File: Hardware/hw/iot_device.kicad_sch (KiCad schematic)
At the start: 38 parts, among them J2 USB4085-GF-A_REVA4, J4 Conn_01x04_Pin, J7 Conn_01x02_Pin, Q1 PMOS, Q7 PMOS, SW1 SW_Push, SW2 SW_Push, U1 ESP32-C6-WROOM-1, U2 RV-3028-C7, U5 TPS63001, U9 USBLC6-4SC6

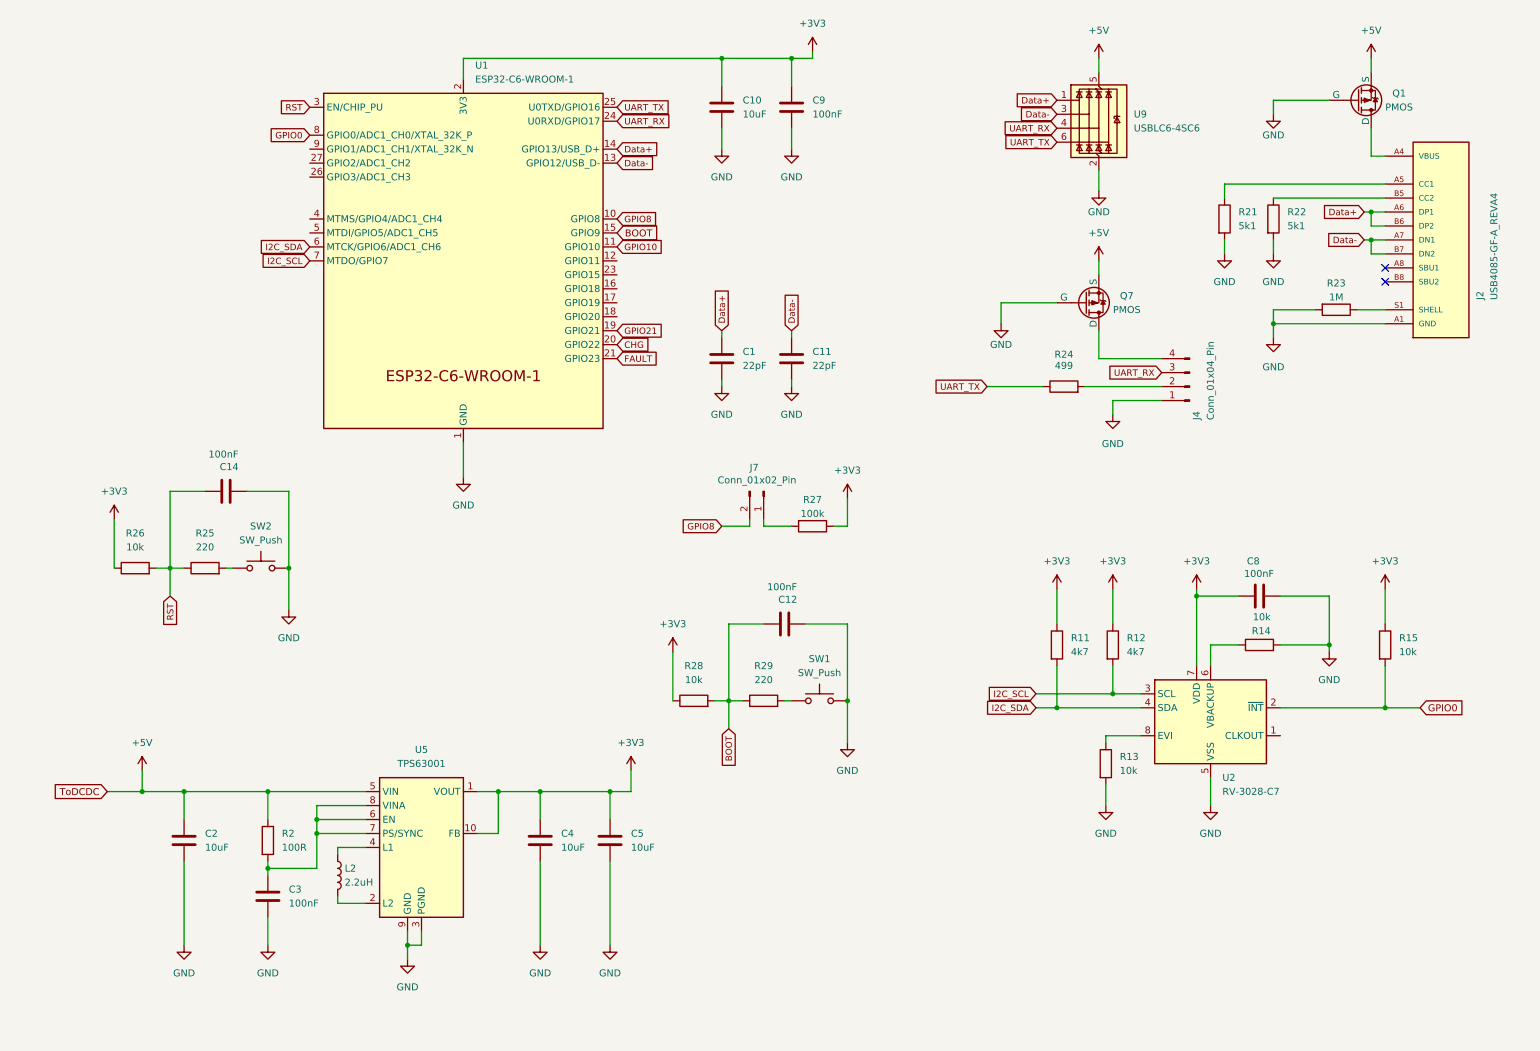
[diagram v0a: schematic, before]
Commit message: Sensors update
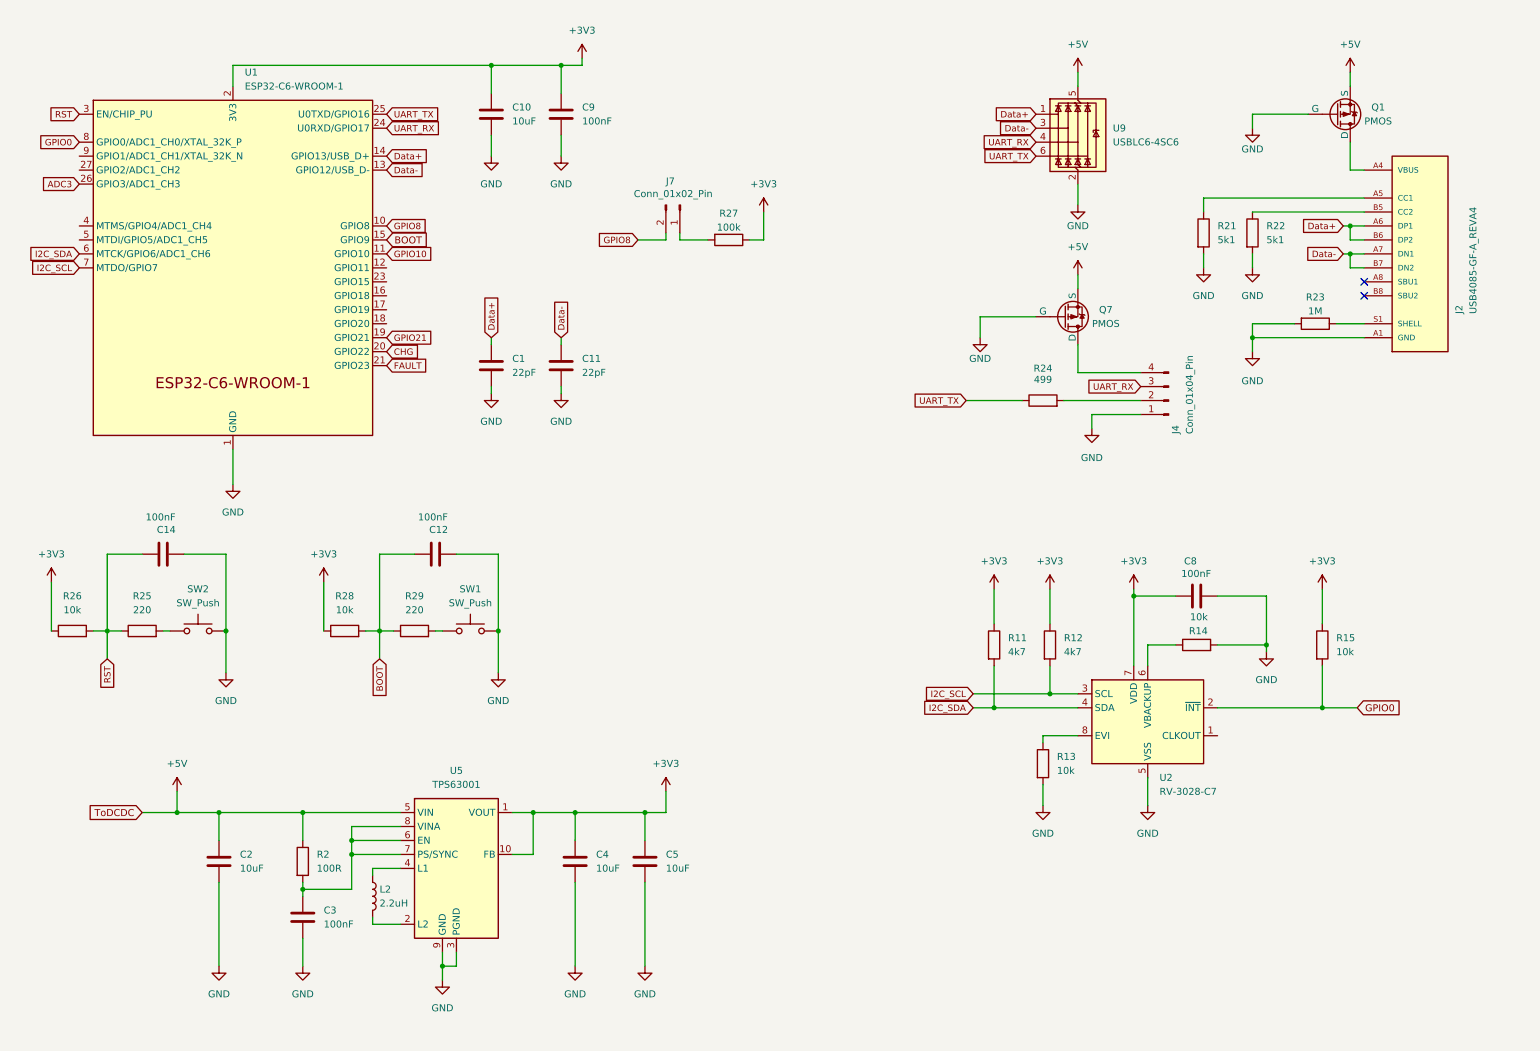
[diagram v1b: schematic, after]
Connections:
- net ADC3: now reaches U1.26 (GPIO3/ADC1_CH3)
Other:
- moved on the sheet: C1, C10, C11, C12, C14, C2, C3, C4, C5, C8, C9, J2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

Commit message: Hardware v1.0
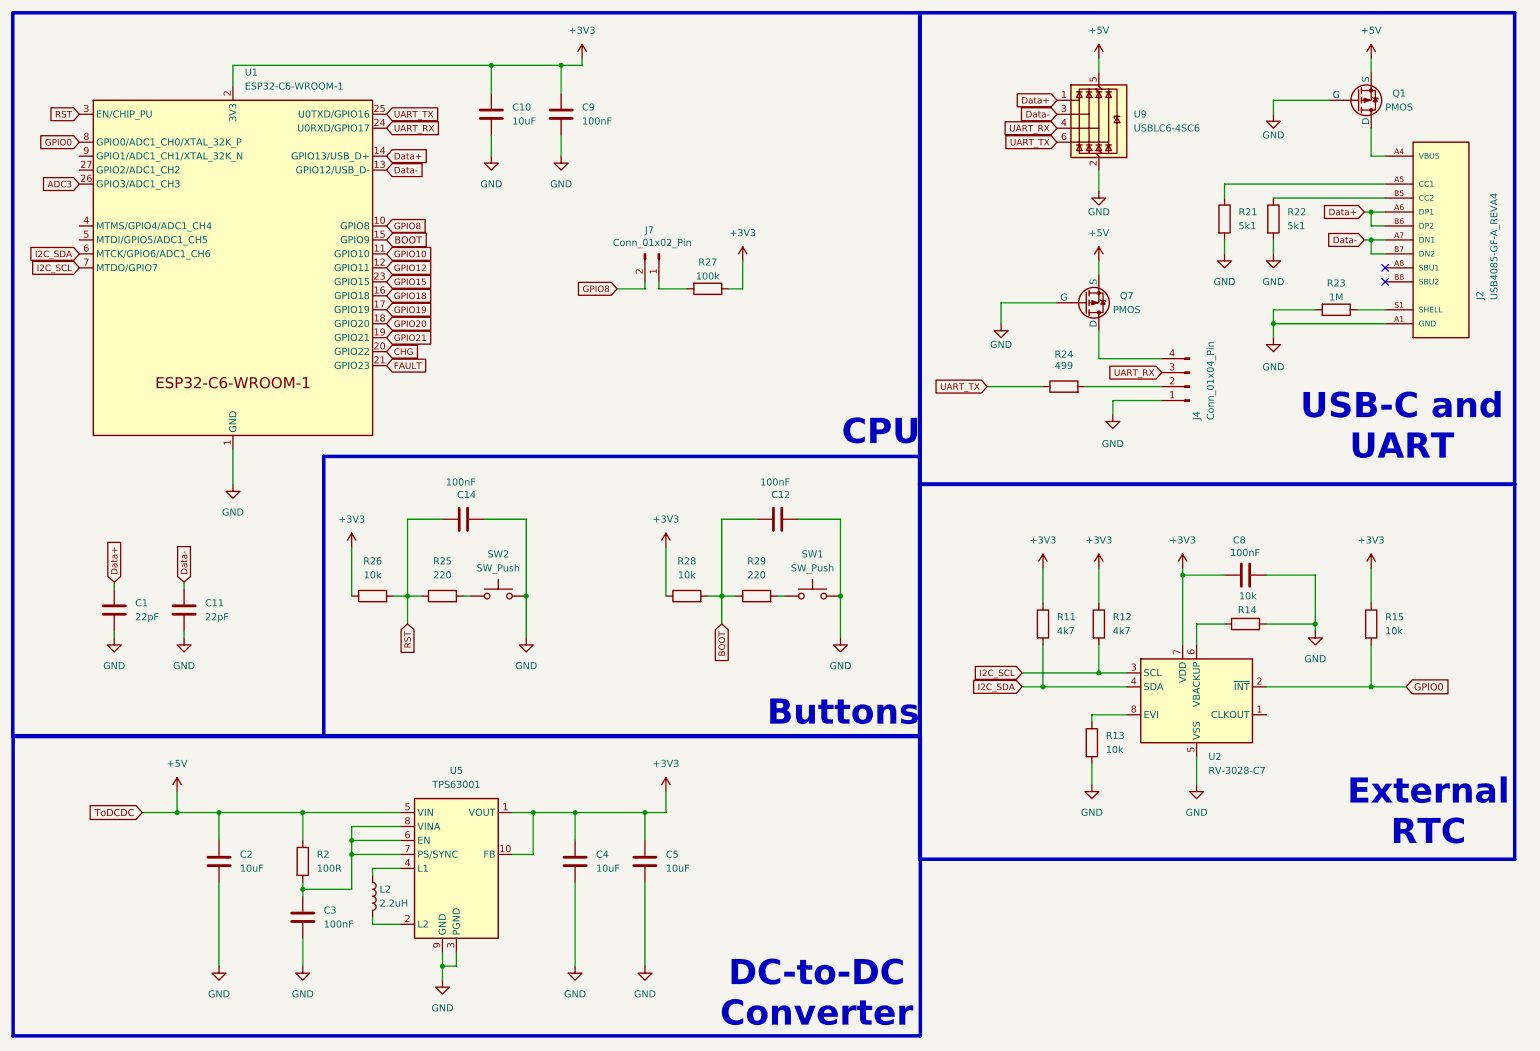
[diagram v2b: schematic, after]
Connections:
- net GPIO12: now reaches U1.12 (GPIO11)
- net GPIO18: now reaches U1.16 (GPIO18)
- net GPIO19: now reaches U1.17 (GPIO19)
- net GPIO20: now reaches U1.18 (GPIO20)
- net GPIO15: now reaches U1.23 (GPIO15)
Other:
- note added: "Buttons"
- note added: "CPU"
- note added: "DC-to-DC Converter"
- note added: "External RTC"
- note added: "USB-C and UART"
- company: (none) -> UNIZA Faculty of Management Science and Informatics Department of Technical Cybernetics
- title: (none) -> Solar Power Management and Monitoring Circuit
- moved on the sheet: C1, C11, C12, C14, C8, J2, J4, J7, Q1, Q7, R11, R12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
